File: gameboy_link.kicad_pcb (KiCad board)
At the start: 2 copper layers, 15.3 x 21.3 mm, 3 parts, among them J1 M5StickC Connector, U1 GameBoy_Link

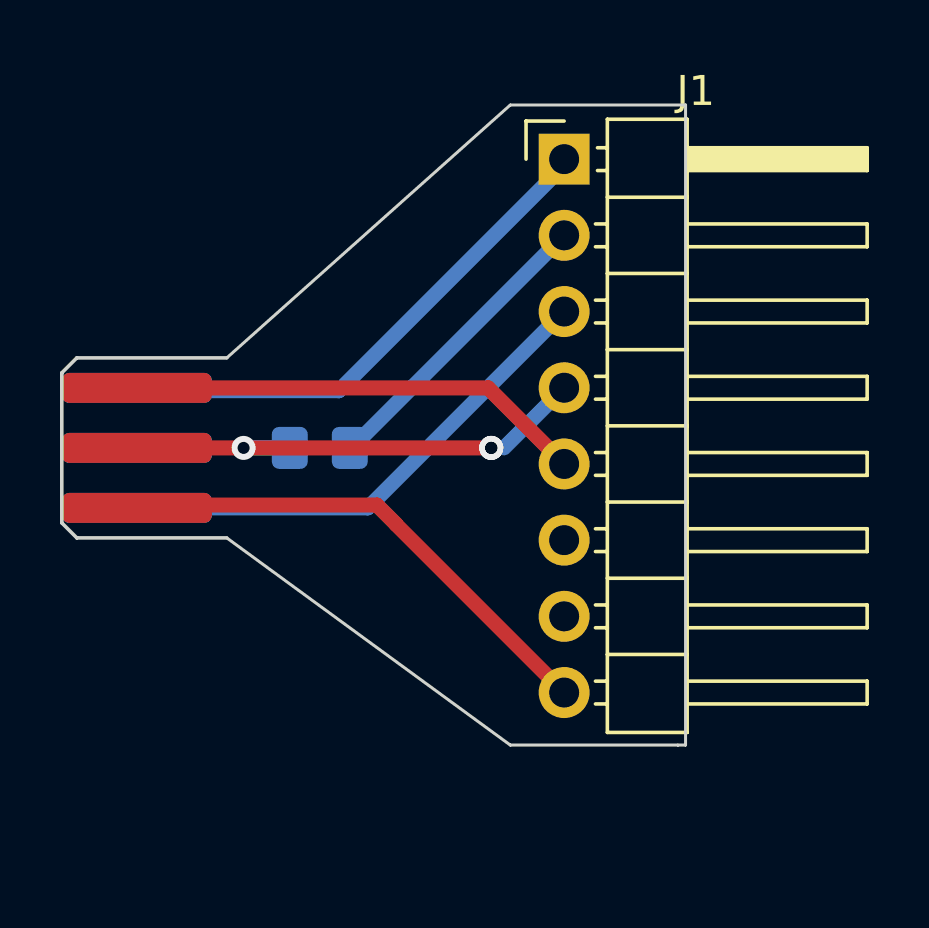
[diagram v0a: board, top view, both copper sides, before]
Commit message: update desgin
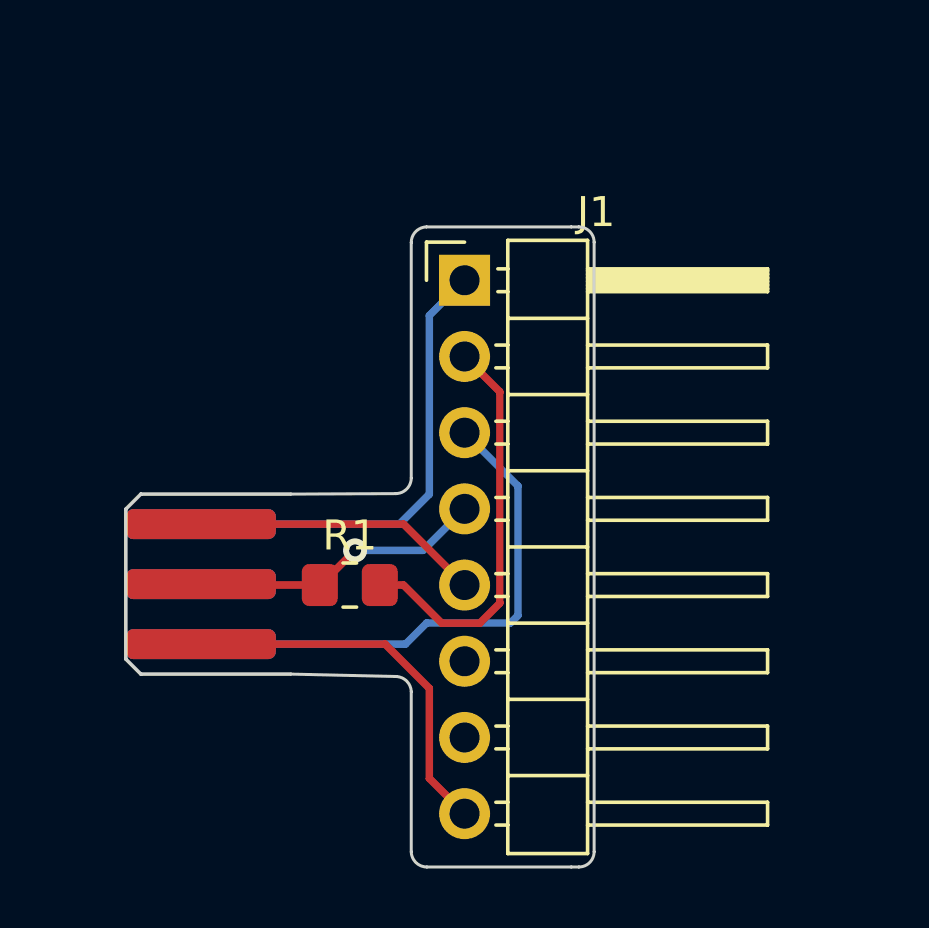
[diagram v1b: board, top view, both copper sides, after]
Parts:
- R1: moved to F.Cu
- moved J1 5.23 mm to (154.7, 94.7)
- moved U1 5.02 mm to (143.4, 102.4)
- moved R1 4.68 mm to (150.9, 104.9)
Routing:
- net Sck: track 15.3 -> 8.36 mm
- net Sin: track 16.6 -> 9.86 mm, vias 3 -> 1
- net Vcc: track 16.9 -> 11.6 mm
- net Net-(J1-Pad2): track 10.1 -> 13.5 mm
- net GND: track 17.6 -> 14.4 mm
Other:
- board size 15.3 x 21.3 mm -> 10.1 x 21.3 mm
- board text added: "M5StickC GameBoy Link V1"
